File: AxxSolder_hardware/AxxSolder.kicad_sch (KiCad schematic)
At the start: 150 parts, among them IC1 TLV76733DRVR, IC2 OPA2387DSGT, IC3 LMR54406DBVR, IC4 STM32G431CBT6, IC5 TPD4E1U06DBVR, IC6 STUSB4500QTR, IC7 MAX16171ATA_VY+T, IC8 LTC4440AHMS8E, IC9 INA281A5QDBVRQ1, J1 USB4110-GF-A, J2 691243110009, J3 TSW-102-07-T-S, J4 61300611821, J5 TSW-102-07-T-S, J6 TSW-102-07-T-S, J7 TSW-108-07-T-S, J8 Conn_01x01_Pin, Q1 STL9P3LLH6, Q2 STL10N3LLH5, Q3 2N7002NXAKR, U2 PEC11J-9215F-S0015, U3 BSC014N04LS

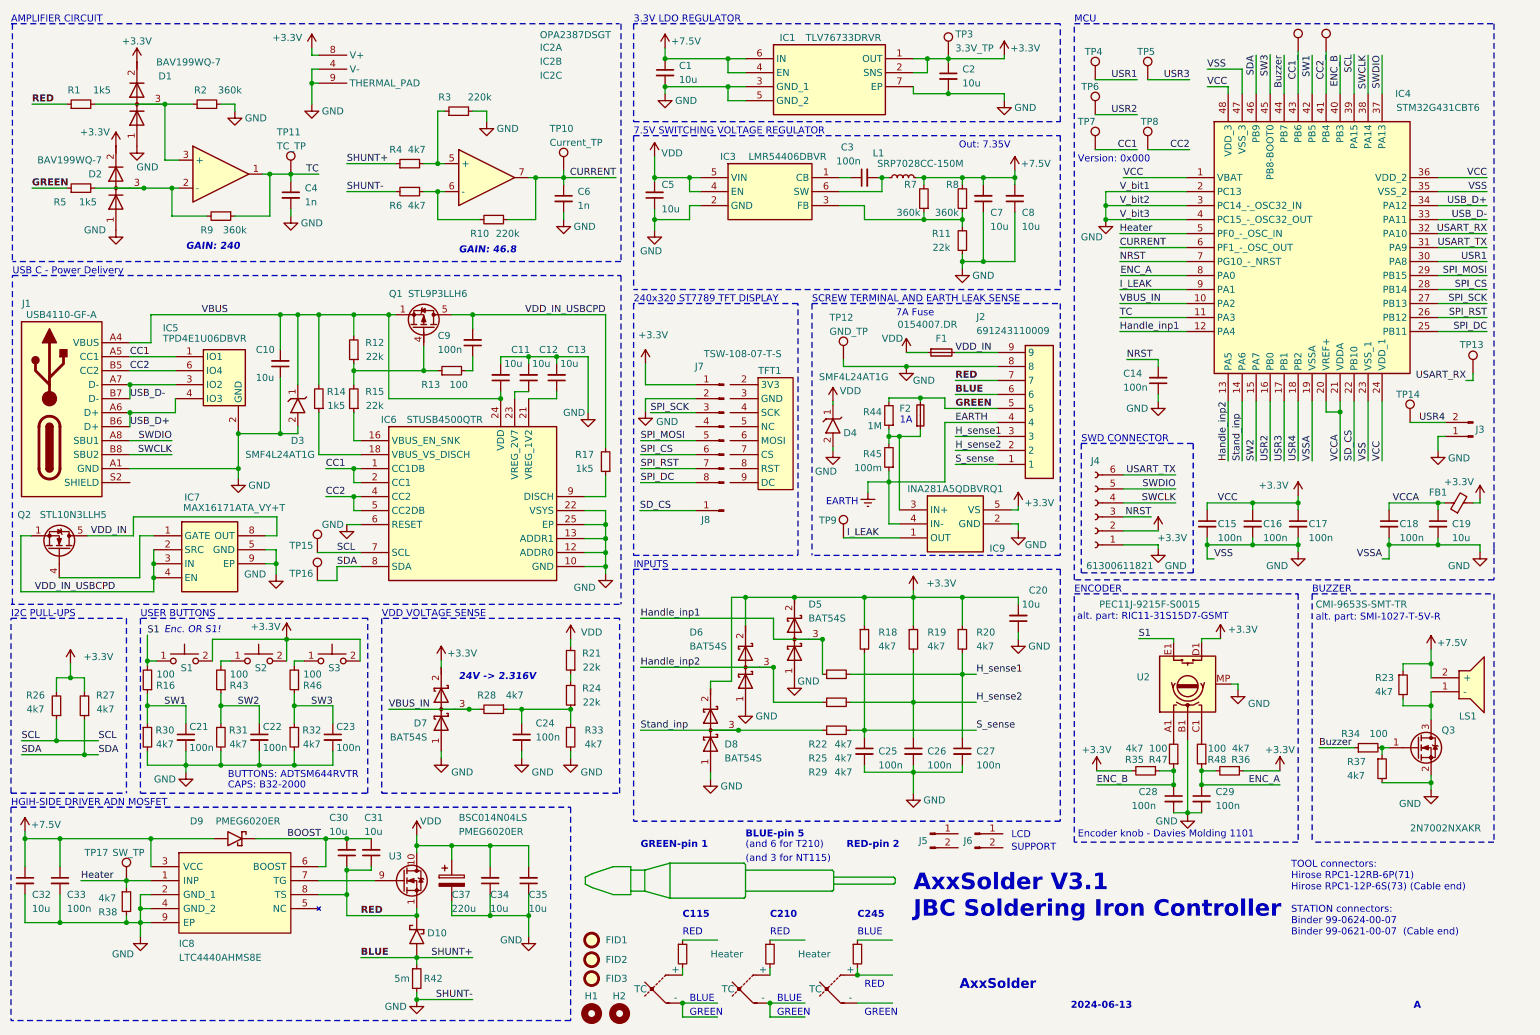
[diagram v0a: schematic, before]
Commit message: Actualización Esquema y PCB
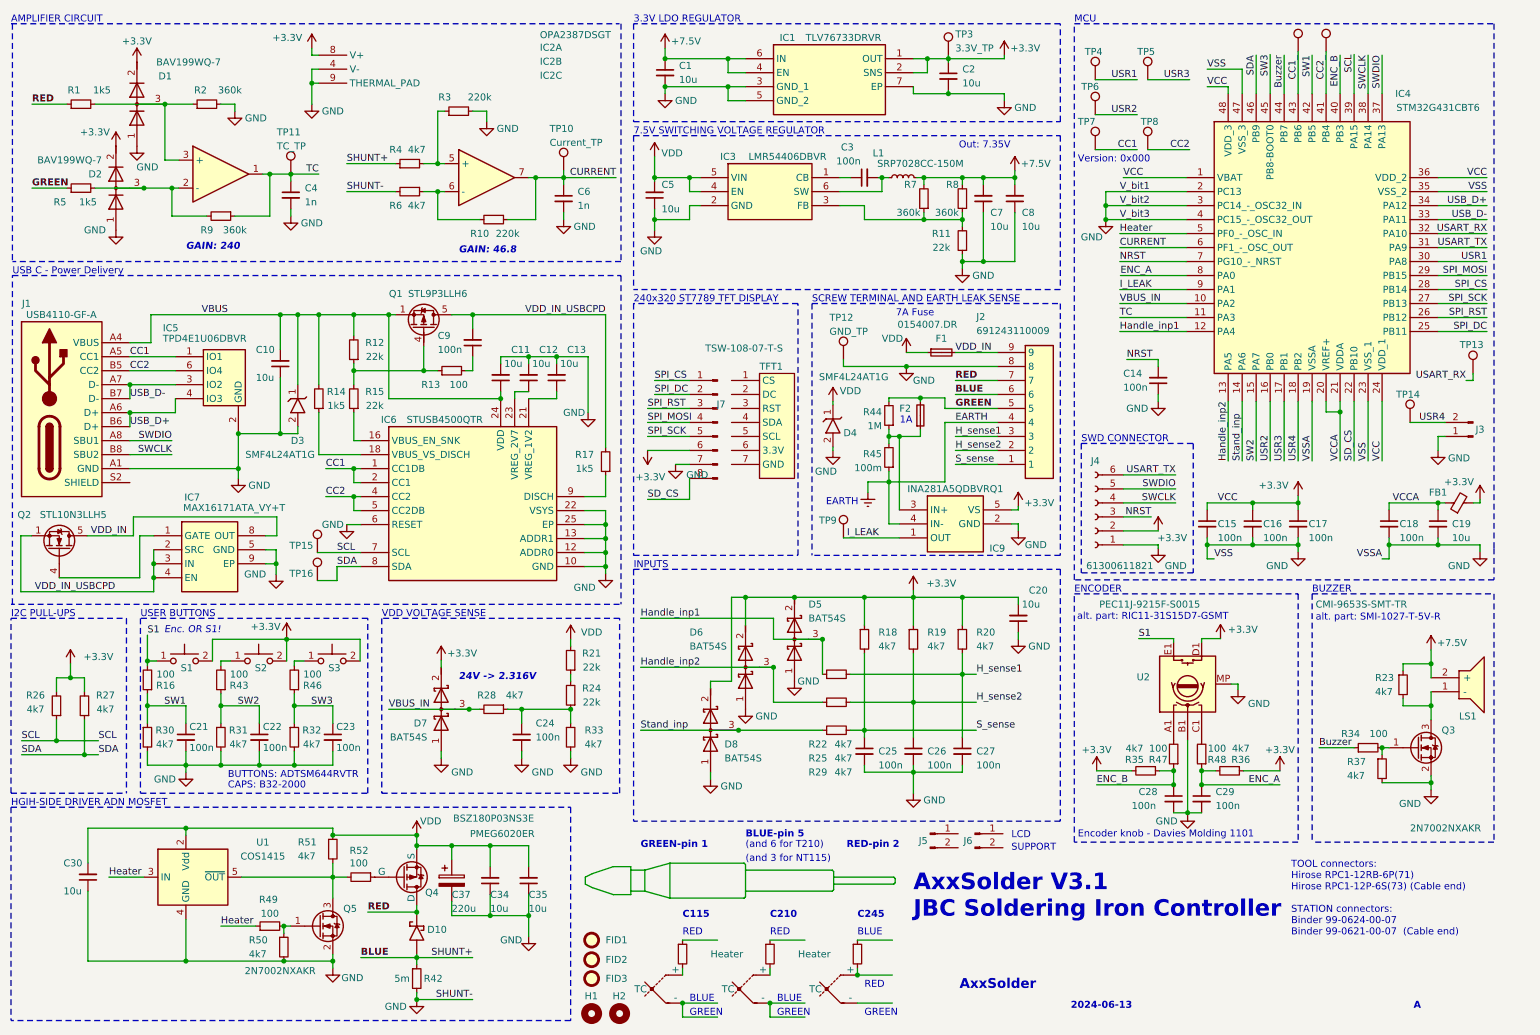
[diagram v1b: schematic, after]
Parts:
- removed C31, C32: 10u, Capacitor_SMD:C_0603_1608Metric, symbol Device:C_Small
- removed C33: 100n, Capacitor_SMD:C_0603_1608Metric, symbol Device:C_Small
- removed D9: PMEG6020ER, footprints:PMEG6020ER115, symbol PMEG6020ER_115:PMEG6020ER,115
- removed IC8: LTC4440AHMS8E, footprints:SOP65P490X110-9N, symbol LTC4440AHMS8E-5#PBF:LTC4440AHMS8E-5#PBF
- removed J8: Conn_01x01_Pin, symbol Connector:Conn_01x01_Pin
- removed R38: 4k7, Resistor_SMD:R_0603_1608Metric, symbol Device:R_Small
- removed TP17: SW_TP, TestPoint:TestPoint_Pad_D1.0mm, symbol Connector:TestPoint
- removed U3: BSC014N04LS, footprints:BSC014N04LS, symbol BSC014N04LS:BSC014N04LS
- added Q4: BSZ180P03NS3E, Package_TO_SOT_SMD:TDSON-8-1, symbol Simulation_SPICE:PMOS
- added Q5: 2N7002NXAKR, footprints:SOT95P230X110-3N, symbol 2N7002NXAKR:2N7002NXAKR
- added R49, R52: 100, Resistor_SMD:R_0603_1608Metric, symbol Device:R_Small
- added R50: 4k7, Resistor_SMD:R_0603_1608Metric, symbol Device:R_Small
- added R51: 4k7, Resistor_SMD:R_1210_3225Metric_Pad1.30x2.65mm_HandSolder, symbol Device:R_Small
- added U1: COS1415, Package_TO_SOT_SMD:SOT-23-5, symbol Driver_FET:MCP1415
- IC2: footprint footprints:SON50P200X200X80-9N -> Package_SO:VSSOP-8_3x3mm_P0.65mm
- J7: symbol TSW-108-07-T-S:TSW-108-07-T-S -> Connector:Conn_01x08_Pin
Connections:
- net BOOST is gone; now on net VDD: C30.2
- net +3.3V: now also J7.6 (Pin_6); no longer J7.1 (Pin_1)
- net GND: now also C30.1, J7.7 (Pin_7), Q5.2 (S), R50.2, U1.4 (GND); no longer J7.2 (Pin_2)
- net Heater: now also R49.1, U1.3 (IN)
- net RED: now also Q4.5 (D); no longer C30.1
- net SD_CS: now also J7.8 (Pin_8)
- net SPI_CS: now also J7.1 (Pin_1); no longer J7.6 (Pin_6)
- net SPI_DC: now also J7.2 (Pin_2); no longer J7.8 (Pin_8)
- net SPI_MOSI: now also J7.4 (Pin_4); no longer J7.5 (Pin_5)
- net SPI_RST: now also J7.3 (Pin_3); no longer J7.7 (Pin_7)
- net SPI_SCK: now also J7.5 (Pin_5); no longer J7.3 (Pin_3)
- net VDD: now also Q4.1 (S), R51.1, U1.2 (Vdd)
- new net: Q4.4 (G), R52.1
- new net: Q5.3 (D), R51.2, R52.2, U1.5 (~{OUT})
- new net: Q5.1 (G), R49.2, R50.1
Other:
- moved on the sheet: D10, J7
